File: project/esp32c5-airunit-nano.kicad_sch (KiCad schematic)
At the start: 26 parts, among them J1 FPC0.5B-WTX-24P, J2 Conn_01x01_Pin, J4 Conn_01x01_Pin, J5 Conn_01x01_Pin, J6 Conn_01x01_Pin, J7 Conn_01x01_Pin, J8 TF-021B-H265, J9 Conn_01x01_Pin, SW1 EVQP7C01P, U1 MT3406, U2 ESP32-C5-WROOM-1U-N8R8, Y1 YD24MUBCE2O

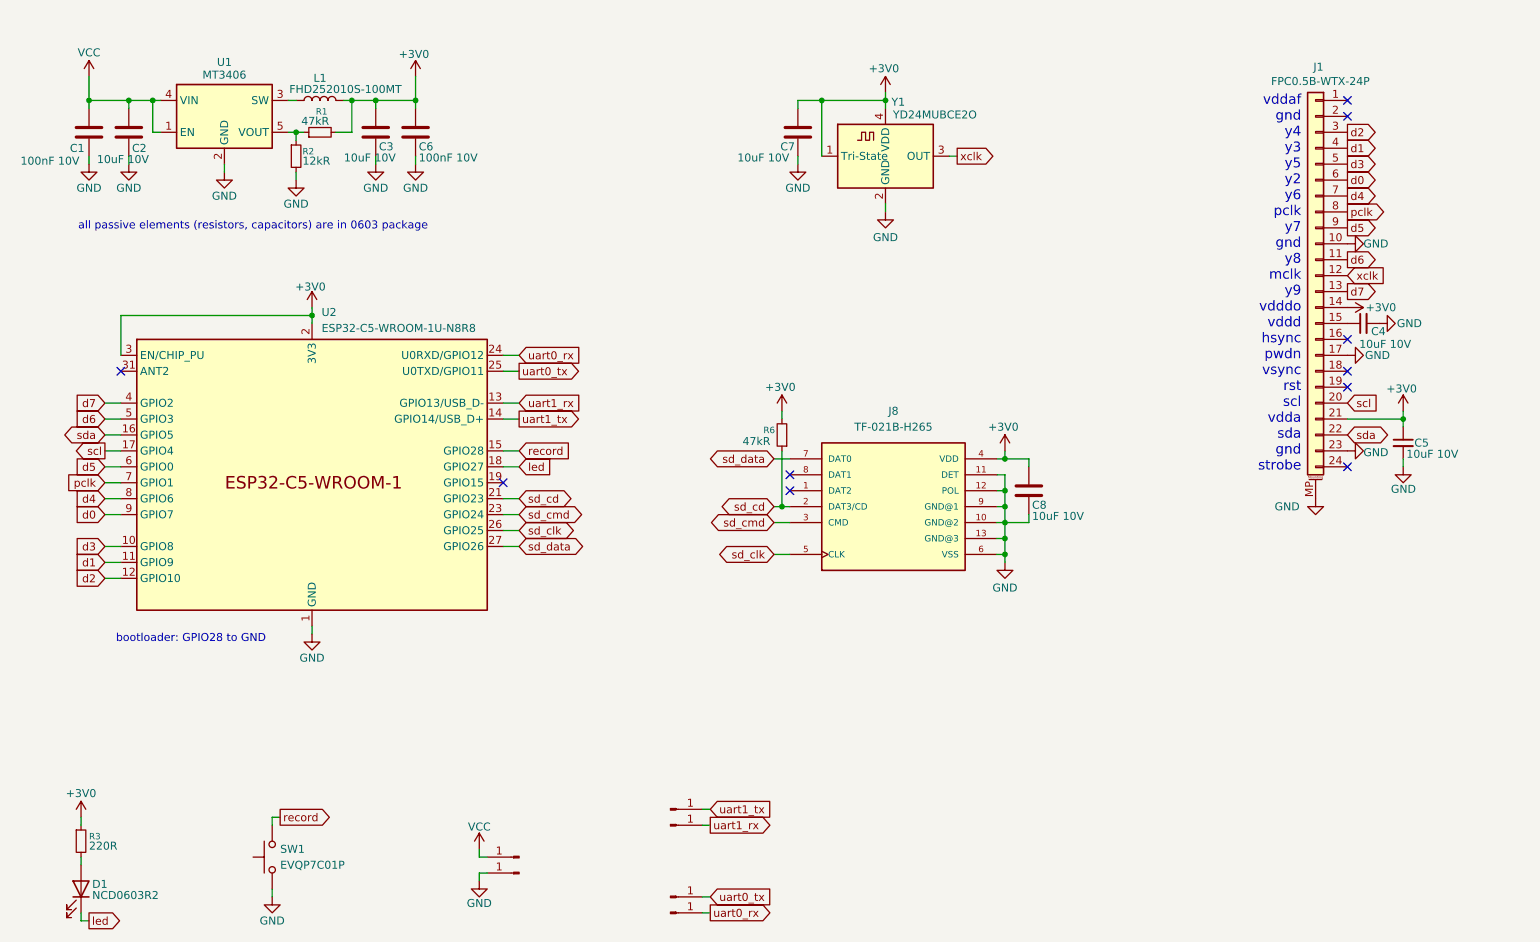
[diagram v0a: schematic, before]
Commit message: i've uploaded the v1.2
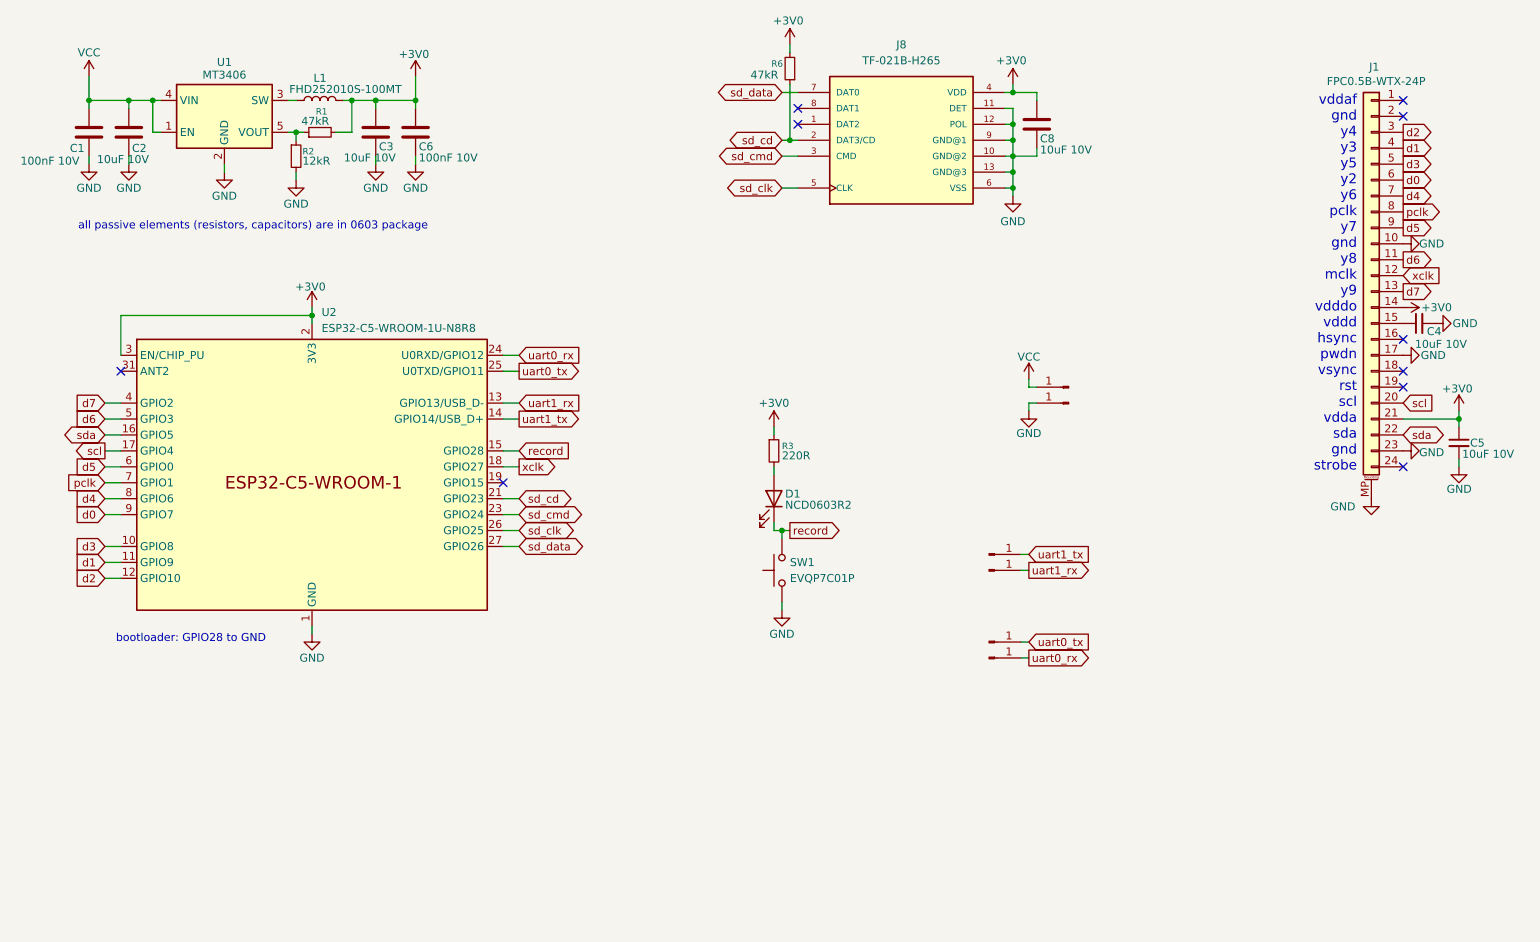
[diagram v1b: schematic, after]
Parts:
- removed C7: 10uF 10V, Capacitor_SMD:C_0603_1608Metric, symbol Device:C
- removed Y1: YD24MUBCE2O, Oscillator:Oscillator_SMD_ECS_2520MV-xxx-xx-4Pin_2.5x2.0mm, symbol Oscillator:ECS-2520MV-xxx-xx
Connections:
- net record: now also D1.1 (K)
- net xclk: now also U2.18 (GPIO27)
- removed net led: D1.1 (K), U2.18 (GPIO27)
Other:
- moved on the sheet: C4, C5, C8, D1, J1, J8, R3, R6, SW1
